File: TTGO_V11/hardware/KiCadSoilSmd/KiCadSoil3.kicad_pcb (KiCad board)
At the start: 2 copper layers, 74.9 x 18.4 mm, 11 parts, among them J1 Screw_Terminal_01x03, U1 ATtiny85-20PU, U2 TLC555CD

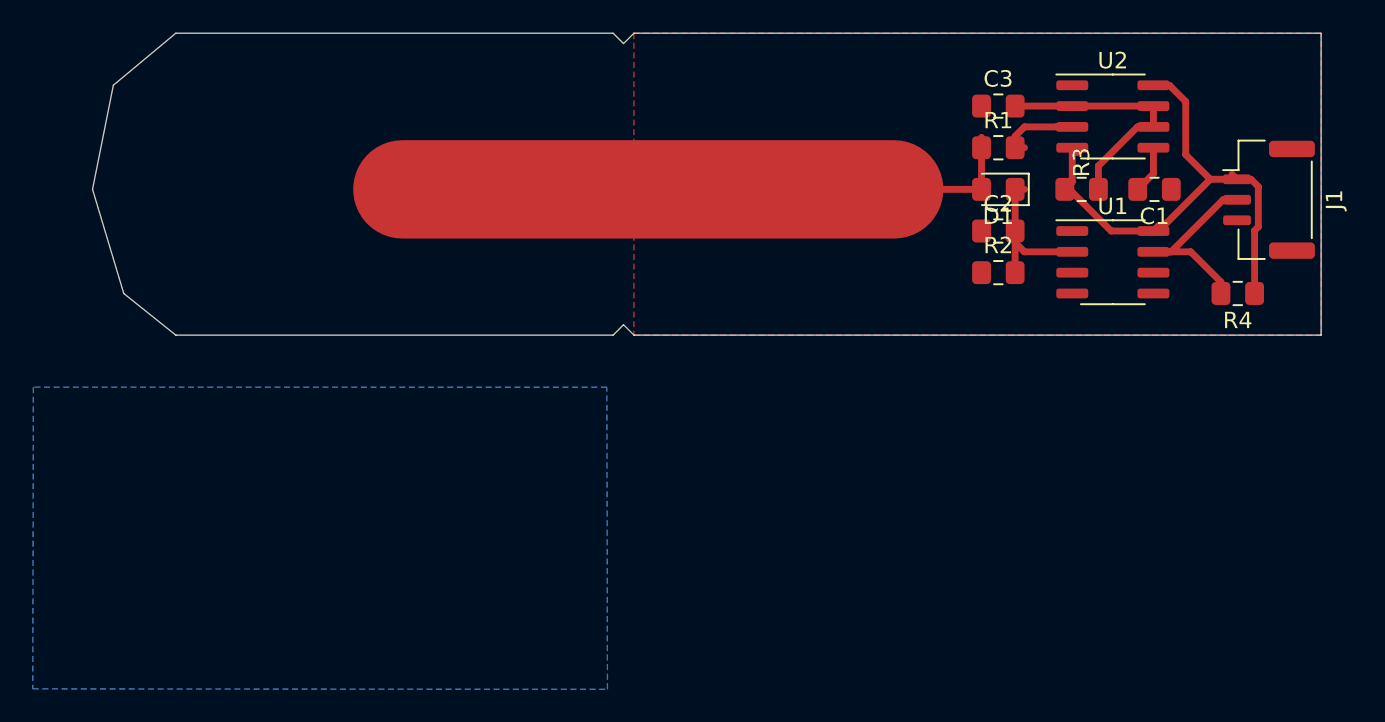
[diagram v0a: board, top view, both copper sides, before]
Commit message: board changes
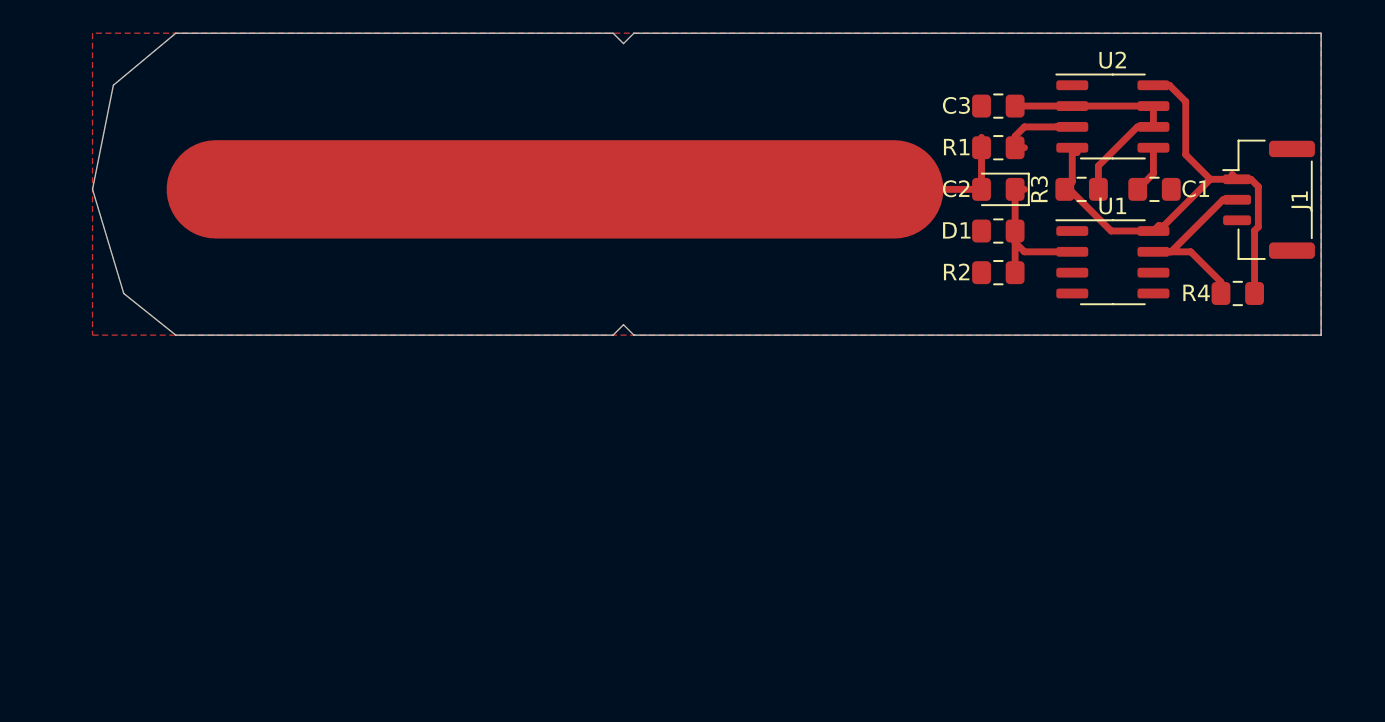
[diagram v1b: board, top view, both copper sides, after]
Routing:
- net /COUT: track 38.5 -> 49.9 mm
- removed copper zone on B.Cu, net GND
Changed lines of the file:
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@@
     (tags "connector JST GH side entry")
     (attr smd)
-    (fp_text reference J1 (at 0 -4 90) (layer F.SilkS)
-      (effects (font (size 1 1) (thickness 0.15)))
-    )
-    (fp_text value Screw_Terminal_01x03 (at 0 4 90) (layer F.Fab)
+    (fp_text reference J1 (at 0 -1.905 90) (layer F.SilkS)
+      (effects (font (size 1 1) (thickness 0.15)))
+    )
+    (fp_text value Screw_Terminal_01x03 (at 0.635 -5.08 90) (layer F.Fab)
       (effects (font (size 1 1) (thickness 0.15)))
     )
@@
     (tags "diode handsolder")
     (attr smd)
-    (fp_text reference D1 (at 0 -1.65) (layer F.SilkS)
+    (fp_text reference D1 (at 2.54 -2.54) (layer F.SilkS)
       (effects (font (size 1 1) (thickness 0.15)))
     )
@@
     (tags "capacitor handsolder")
     (attr smd)
-    (fp_text reference C3 (at 0 -1.65) (layer F.SilkS)
-      (effects (font (size 1 1) (thickness 0.15)))
-    )
-    (fp_text value 330p (at 0 1.65) (layer F.Fab)
+    (fp_text reference C3 (at -2.54 0) (layer F.SilkS)
+      (effects (font (size 1 1) (thickness 0.15)))
+    )
+    (fp_text value 330p (at -3.175 0) (layer F.Fab)
       (effects (font (size 1 1) (thickness 0.15)))
     )
@@
     (tags "capacitor handsolder")
     (attr smd)
-    (fp_text reference C2 (at 0 -1.65) (layer F.SilkS)
+    (fp_text reference C2 (at -2.54 -2.54) (layer F.SilkS)
       (effects (font (size 1 1) (thickness 0.15)))
     )
@@
     (tags "capacitor handsolder")
     (attr smd)
-    (fp_text reference C1 (at 0 -1.65) (layer F.SilkS)
+    (fp_text reference C1 (at -2.54 0) (layer F.SilkS)
       (effects (font (size 1 1) (thickness 0.15)))
     )
@@
     (tags "resistor handsolder")
     (attr smd)
-    (fp_text reference R4 (at 0 -1.65) (layer F.SilkS)
+    (fp_text reference R4 (at 2.54 0) (layer F.SilkS)
       (effects (font (size 1 1) (thickness 0.15)))
     )
@@
     (tags "resistor handsolder")
     (attr smd)
-    (fp_text reference R3 (at 0 -1.65 90) (layer F.SilkS)
+    (fp_text reference R3 (at -2.54 0 90) (layer F.SilkS)
       (effects (font (size 1 1) (thickness 0.15)))
     )
@@
     (tags "resistor handsolder")
     (attr smd)
-    (fp_text reference R2 (at 0 -1.65) (layer F.SilkS)
+    (fp_text reference R2 (at -2.54 0) (layer F.SilkS)
       (effects (font (size 1 1) (thickness 0.15)))
     )
@@
     (tags "resistor handsolder")
     (attr smd)
-    (fp_text reference R1 (at 0 -1.65) (layer F.SilkS)
-      (effects (font (size 1 1) (thickness 0.15)))
-    )
-    (fp_text value 10k (at 0 1.65) (layer F.Fab)
+    (fp_text reference R1 (at -2.54 0) (layer F.SilkS)
+      (effects (font (size 1 1) (thickness 0.15)))
+    )
+    (fp_text value 10k (at -2.54 0) (layer F.Fab)
       (effects (font (size 1 1) (thickness 0.15)))
     )
@@
   (segment (start 91.83 41.91) (end 91.83 40.48) (width 0.42) (layer F.Cu) (net 7))
   (segment (start 90.235 36.83) (end 86.75 36.83) (width 0.42) (layer F.Cu) (net 7))
-  (segment (start 49.375 41.91) (end 79.375 41.91) (width 6) (layer F.Cu) (net 8))
+  (segment (start 38 41.91) (end 79.375 41.91) (width 6) (layer F.Cu) (net 8))
   (segment (start 84.7 38.735) (end 84.7 41.91) (width 0.42) (layer F.Cu) (net 8))
   (segment (start 84.7 41.91) (end 79.375 41.91) (width 0.42) (layer F.Cu) (net 8))
@@
     (polygon
       (pts
-        (xy 105.41 32.385) (xy 63.5 32.385) (xy 63.5 50.8) (xy 105.41 50.8)
+        (xy 105.41 32.385) (xy 30.48 32.385) (xy 30.48 50.8) (xy 105.41 50.8)
       )
     )
-  )
-  (zone (net 2) (net_name GND) (layer B.Cu) (hatch edge 0.508)
-    (connect_pads yes (clearance 1.9))
-    (min_thickness 1)
-    (fill yes (arc_segments 32) (thermal_gap 1) (thermal_bridge_width 1.1))
-    (polygon
-      (pts
-        (xy 61.849782 53.975524) (xy 26.871054 53.971621) (xy 26.836187 72.375716) (xy 61.884649 72.401428)
-      )
-    )
